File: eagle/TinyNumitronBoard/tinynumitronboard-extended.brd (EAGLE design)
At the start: 100 x 50 mm, 51 parts

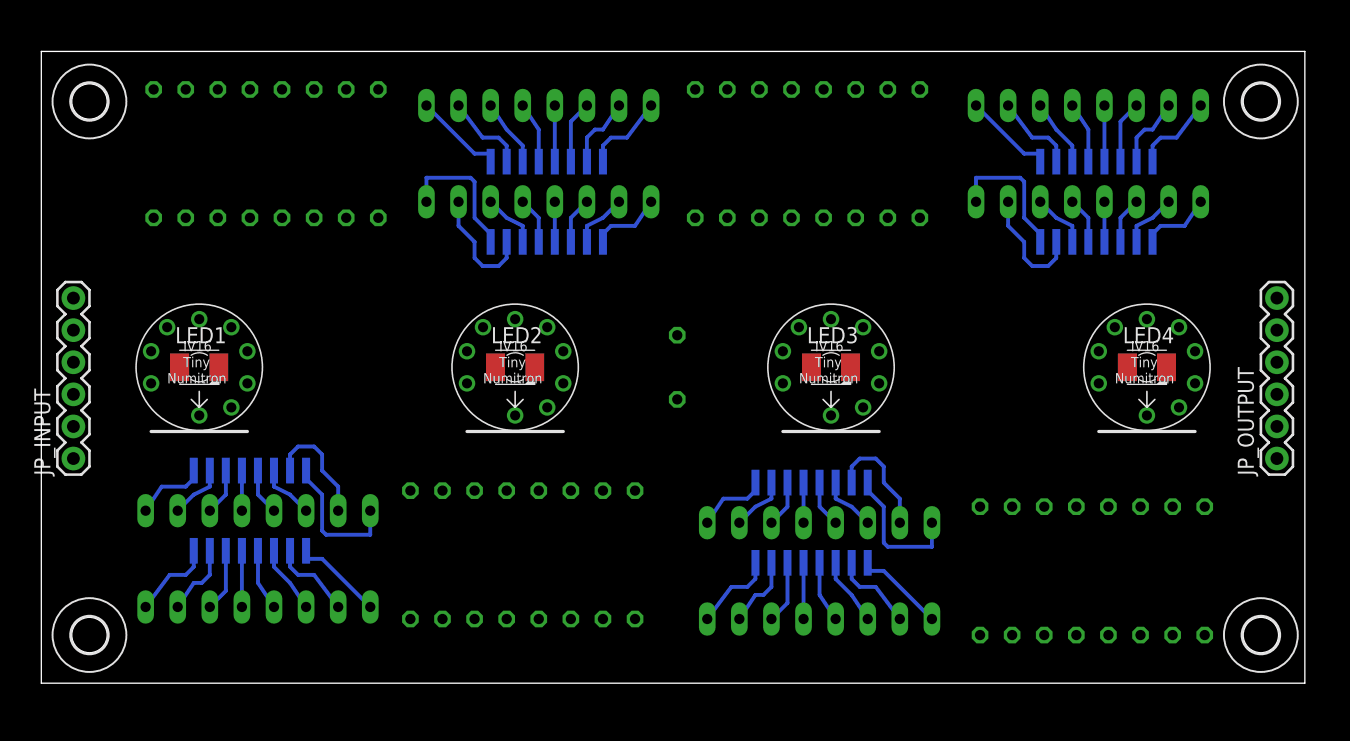
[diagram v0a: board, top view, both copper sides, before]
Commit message: Version 1.0 sent to production with nice image on the top.
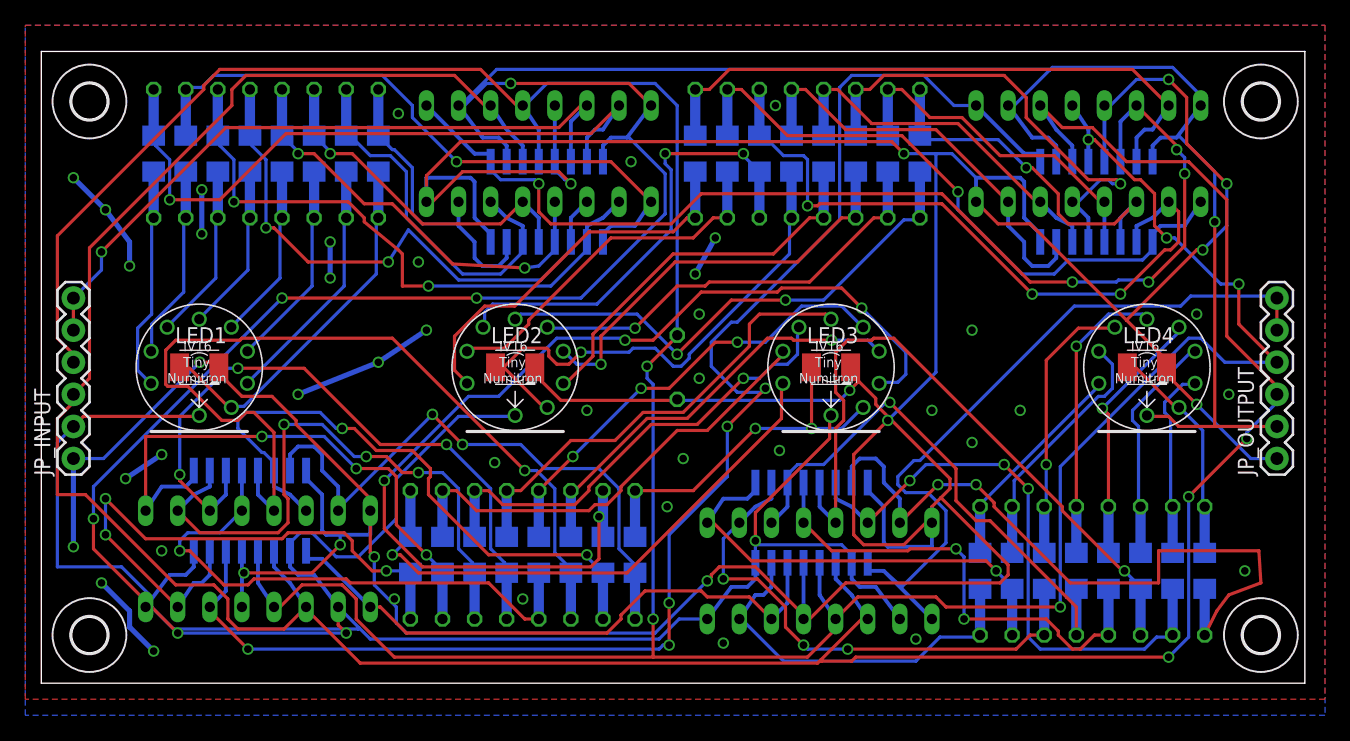
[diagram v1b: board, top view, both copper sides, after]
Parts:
- added U$3: (no value), kalshagar-images:GEARS_1000X500
- R1, R10, R11, R12, R13, R14, R15, R16, R17, R18, R19, R2, R20, R21, R22, R23, R24, R25, R26, R27, R28, R29, R3, R30, R31, R32, R4, R5, R6, R7, R8, R9: value (none) -> RESISTOR_COMBO1206; device resistor:0207/10 -> kalshagar:207-10_SMD_COMBO
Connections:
- net N$1: now also R1.3
- net N$10: now also R3.4
- net N$11: now also R4.4
- net N$12: now also R5.4
- net N$13: now also R6.4
- net N$14: now also R7.4
- net N$16: now also R8.4
- net N$17: now also R8.3
- net N$2: now also R2.3
- net N$20: now also R9.3
- net N$21: now also R10.3
- net N$24: now also R11.3
- net N$25: now also R12.3
- net N$26: now also R13.3
- net N$27: now also R14.3
- net N$28: now also R15.3
- net N$29: now also R9.4
- net N$3: now also R3.3
- net N$30: now also R10.4
- net N$31: now also R11.4
- net N$32: now also R12.4
- net N$33: now also R13.4
- net N$34: now also R14.4
- net N$35: now also R15.4
- net N$36: now also R16.4
- net N$37: now also R16.3
- net N$39: now also R17.3
- net N$4: now also R4.3
- net N$40: now also R18.3
- net N$41: now also R19.3
- net N$42: now also R20.3
- net N$43: now also R21.3
- net N$44: now also R22.3
- net N$45: now also R23.3
- net N$46: now also R17.4
- net N$47: now also R18.4
- net N$48: now also R19.4
- net N$49: now also R20.4
- net N$5: now also R5.3
- net N$50: now also R21.4
- net N$51: now also R22.4
- net N$52: now also R23.4
- net N$53: now also R24.4
- net N$54: now also R24.3
- net N$6: now also R6.3
- net N$62: now also R25.3
- net N$63: now also R26.3
- net N$64: now also R27.3
- net N$65: now also R28.3
- net N$66: now also R29.3
- net N$67: now also R30.3
- net N$68: now also R31.3
- net N$69: now also R25.4
- net N$7: now also R7.3
- net N$70: now also R26.4
- net N$71: now also R27.4
- net N$72: now also R28.4
- net N$73: now also R29.4
- net N$74: now also R30.4
- net N$75: now also R31.4
- net N$76: now also R32.4
- net N$77: now also R32.3
- net N$8: now also R1.4
- net N$9: now also R2.4
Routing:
- net GND: track 0.00 -> 380.4 mm, vias 0 -> 53
- net VCC: track 0.00 -> 338.2 mm, vias 0 -> 8
- net RCK: track 0.00 -> 242.3 mm, vias 0 -> 6
- net SCK: track 0.00 -> 220.2 mm, vias 0 -> 3
- net N$58: track 0.00 -> 107.4 mm, vias 0 -> 5
- net N$68: track 0.00 -> 81.6 mm, vias 0 -> 4
- net N$23: track 0.00 -> 78.4 mm, vias 0 -> 5
- net N$74: track 0.00 -> 68.4 mm, vias 0 -> 1
- net N$22: track 0.00 -> 53.9 mm
- net N$34: track 0.00 -> 52.6 mm, vias 0 -> 1
- net SER: track 0.00 -> 50.3 mm, vias 0 -> 1
- net N$72: track 0.00 -> 49.4 mm, vias 0 -> 3
- net N$36: track 0.00 -> 48.2 mm, vias 0 -> 2
- net N$48: track 0.00 -> 46.0 mm, vias 0 -> 3
- net N$75: track 0.00 -> 44.8 mm, vias 0 -> 2
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- added copper zone on layer 1, net GND
- added copper zone on layer 16, net GND
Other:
- board text added: "1uF"
- board text added: "74xx595"
- board text added: "Alan numitron clock (v1.0 - July 2013)"
- board text added: "All resistors:100Ω LED:470Ω"
- board text added: "CLK"
- board text added: "DATA(in)"
- board text added: "DATA(out)"
- board text added: "Dot/LED"
- board text added: "GND"
- board text added: "LTCH"
- board text added: "VCC"
- board text added: "[IN]"
- board text added: "[OUT]"
- board text added: "http://kalshagar.wikispaces.com/Alan+numitron+clock"
